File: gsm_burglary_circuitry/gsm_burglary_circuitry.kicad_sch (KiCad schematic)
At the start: 35 parts, among them U1 ESP32-C6-DevKitC-1, U2 PIR_Sensor, U3 LM2596S-ADJ, U4 PIR_Sensor, U5 HC-SR04_Ultrasonic_Sensor, U6 PIR_Sensor, U7 SIM800L-CORE, U8 LM2596S-ADJ

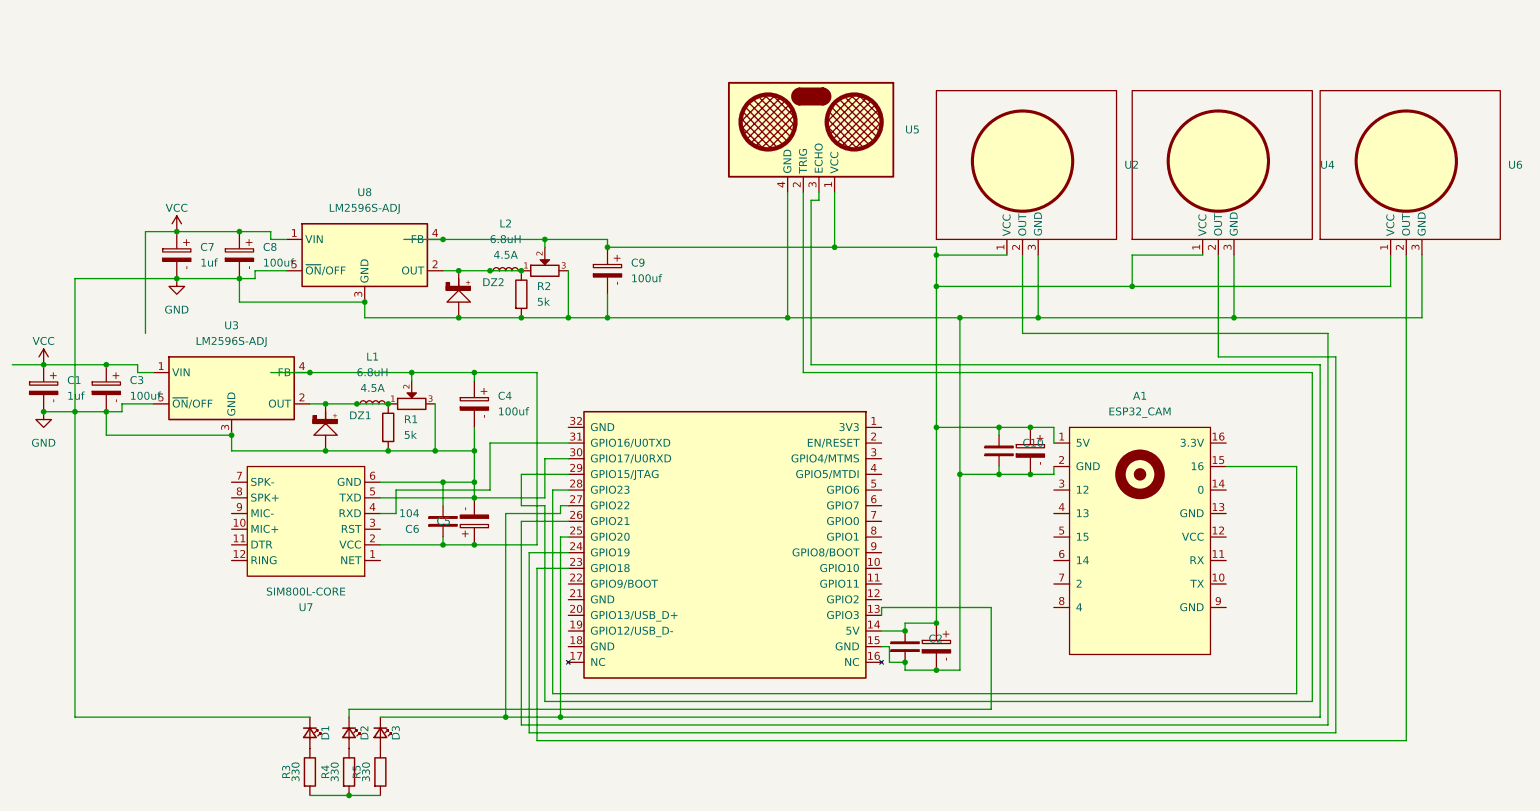
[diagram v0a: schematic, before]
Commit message: made changes
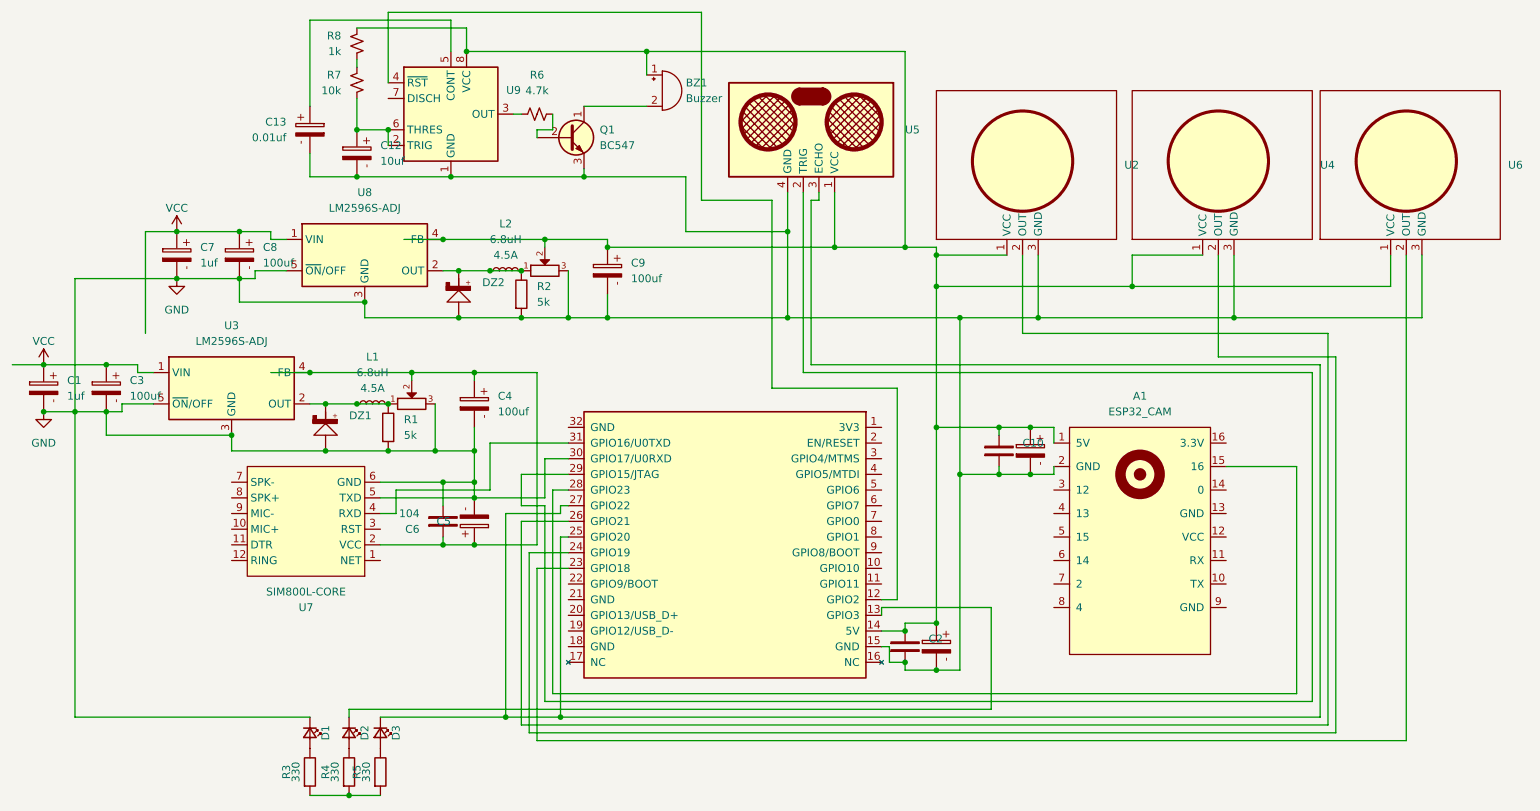
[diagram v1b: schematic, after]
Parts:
- added BZ1: Buzzer, symbol Device:Buzzer
- added C12: 10uf, Capacitor_THT:CP_Radial_D5.0mm_P2.50mm, symbol PCM_SL_Devices:Capacitor_PO
- added C13: 0.01uf, Capacitor_THT:CP_Radial_D5.0mm_P2.50mm, symbol PCM_SL_Devices:Capacitor_PO
- added Q1: BC547, PCM_Package_TO_SOT_THT_AKL:TO-92_Inline_Wide_CBE, symbol PCM_Transistor_BJT_AKL:BC547
- added R6: 4.7k, PCM_SparkFun-Resistor:R_0603_1608Metric, symbol PCM_SparkFun-Resistor:4.7k_0603
- added R7: 10k, PCM_SparkFun-Resistor:R_0603_1608Metric, symbol PCM_SparkFun-Resistor:4.7k_0603
- added R8: 1k, PCM_SparkFun-Resistor:R_0603_1608Metric, symbol PCM_SparkFun-Resistor:4.7k_0603
- added U9: ICM7555xP, Package_DIP:DIP-8_W7.62mm, symbol Timer:ICM7555xP
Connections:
- net GND: now also C12.2, C13.2, Q1.3 (E), U9.1 (GND)
- net at A1.1 (5V), C10.2, C11.1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: now also BZ1.1 (+), R8.2, U9.8 (VCC)
- net at U1.12 (GPIO2): now also U9.4 (~{RST})
- new net: BZ1.2 (-), Q1.1 (C)
- new net: R6.1, U9.3 (OUT)
- new net: Q1.2 (B), R6.2
- new net: C12.1, R7.1, U9.2 (TRIG), U9.6 (THRES)
- new net: C13.1, U9.5 (CONT)
- new net: R7.2, R8.1
